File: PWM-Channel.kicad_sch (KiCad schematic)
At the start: 6 parts, among them U301 TPSM33620S5QRDNRQ1

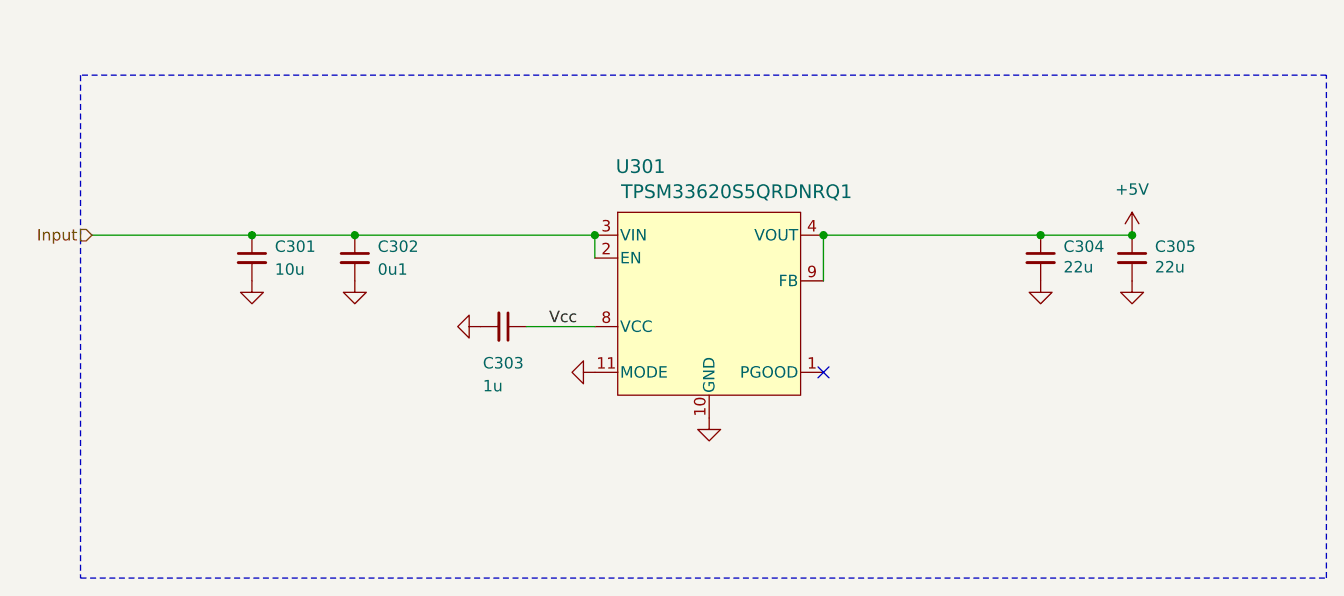
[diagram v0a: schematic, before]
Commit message: Rename
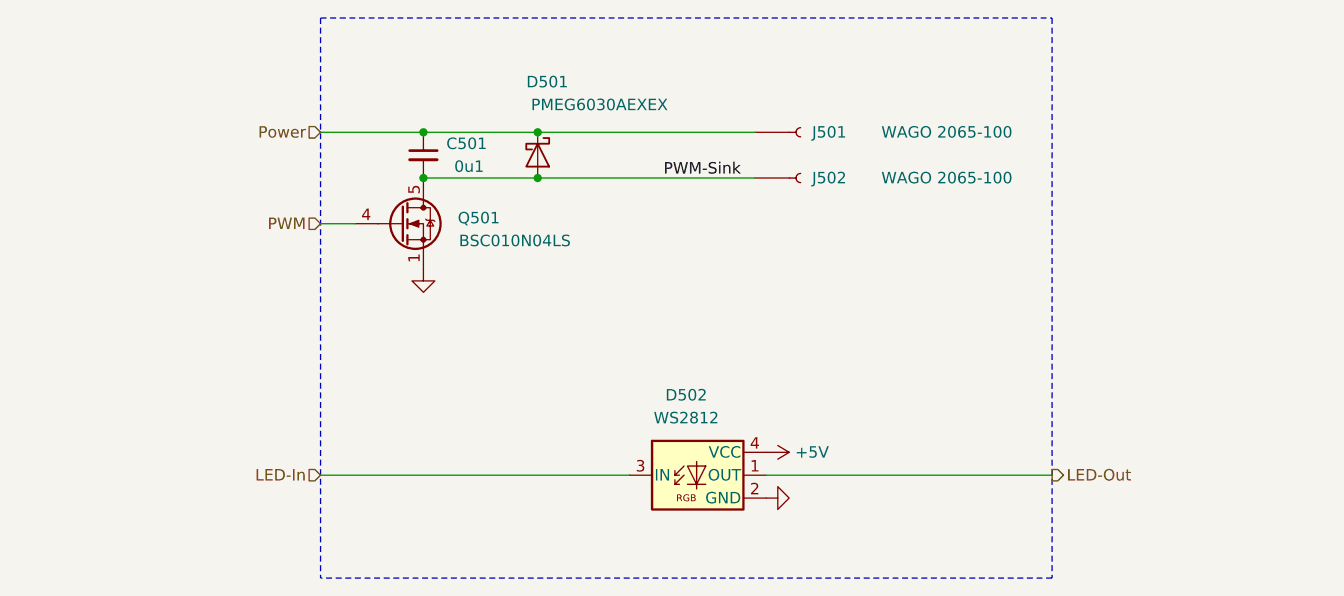
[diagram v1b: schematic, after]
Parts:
- removed C301: 10u, V2_Capacitor_SMD:C_3225, symbol V2_Capacitor:3225_10u
- removed C302: 0u1, V2_Capacitor_SMD:C_1608, symbol V2_Capacitor:1608_0u1
- removed C303: 1u, V2_Capacitor_SMD:C_1608, symbol V2_Capacitor:1608_1u
- removed C304, C305: 22u, V2_Capacitor_SMD:C_3225, symbol V2_Capacitor:3225_22u
- removed U301: TPSM33620S5QRDNRQ1, V2_Converter_DCDC:QFN-11, symbol V2_Converter_DCDC:TPSM33620S5QRDNRQ1
- added C501: 0u1, V2_Capacitor_SMD:C_1608, symbol V2_Capacitor:1608_0u1
- added D501: PMEG6030AEXEX, V2_Diode_SMD:D_SOD-123HP, symbol V2_Diode:PMEG6030AEXEX
- added D502: WS2812, V2_LED:WS2812-2020, symbol V2_LED:WS2812
- added J501, J502: WAGO 2065-100, V2_Connector_WAGO:2065-100, symbol V2_Connector_WAGO:2065
- added Q501: BSC010N04LS, V2_Package_TO_SOT_SMD:TDSON-8-FL, symbol V2_Transistor_FET:BSC010N04LS
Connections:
- net +5V: now also D502.4 (VCC)
- net GND: now also D502.2 (GND), Q501.1 (S)
- new net LED-In: D502.3 (IN)
- new net LED-Out: D502.1 (OUT)
- new net PWM: Q501.4 (G)
- new net PWM-Sink: C501.2, D501.2 (A), J502.1, Q501.5 (D)
- new net Power: C501.1, D501.1 (K), J501.1
- no-connect marks 1 -> 0
